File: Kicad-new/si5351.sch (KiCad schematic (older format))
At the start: 32 parts, among them J11 Link-out 1-0, J12 Link-out 1-0, J13 Link-out 1-1, J14 Link-out 1-1, Q3 BFR92, Q4 BFR92, Q5 BFR92, Q6 BFR92, U6 Si5351A-B-GT, U7 Si5351A-B-GT, Y1 Crystal, Y2 Crystal

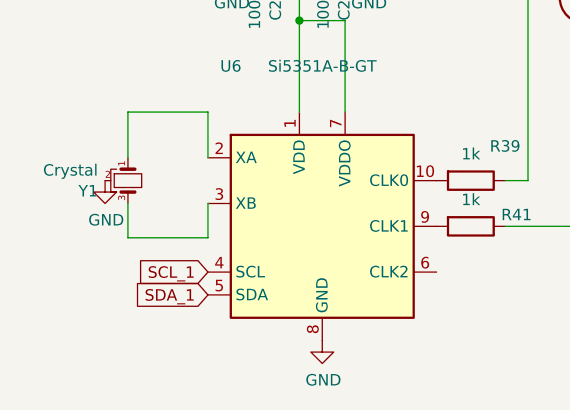
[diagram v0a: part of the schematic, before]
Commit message: new pcb
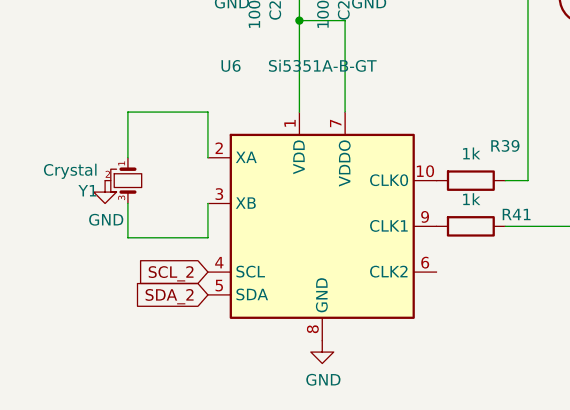
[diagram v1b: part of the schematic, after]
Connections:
- net SCL_1: no longer U6.4 (SCL)
- net SDA_1: no longer U6.5 (SDA)
- new net SCL_2: U6.4 (SCL)
- new net SDA_2: U6.5 (SDA)
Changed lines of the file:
@@
 V33
 Text GLabel 1500 3300 0    50   Input ~ 0
-SDA_1
+SDA_2
 $Comp
 L Connector:Conn_Coaxial J?
@@
 $EndComp
 Text GLabel 1500 3200 0    50   Input ~ 0
-SCL_1
+SCL_2
 $Comp
 L Device:Crystal_GND2_Small Y?
